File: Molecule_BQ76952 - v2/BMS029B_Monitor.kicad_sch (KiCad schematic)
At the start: 108 parts, among them J2 PEC05SAAN, J6 87898-0304, J7 87898-0304, Q1 FCX495TA, U1 bq76952PFBT

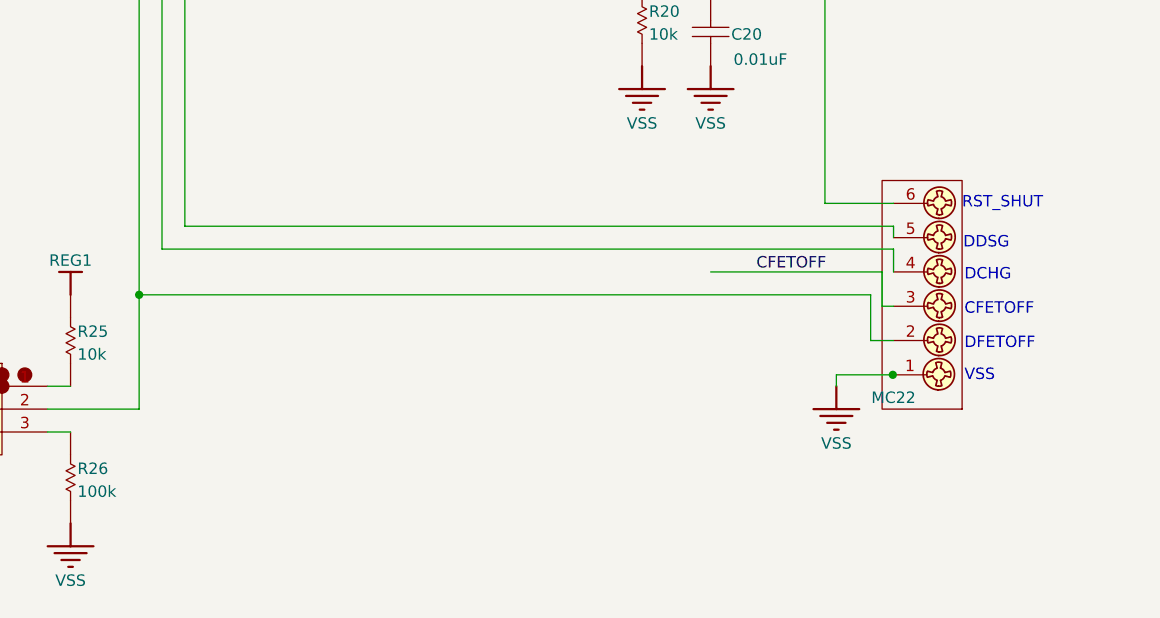
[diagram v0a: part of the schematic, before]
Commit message: Final production
Updated sizing and bug fixes
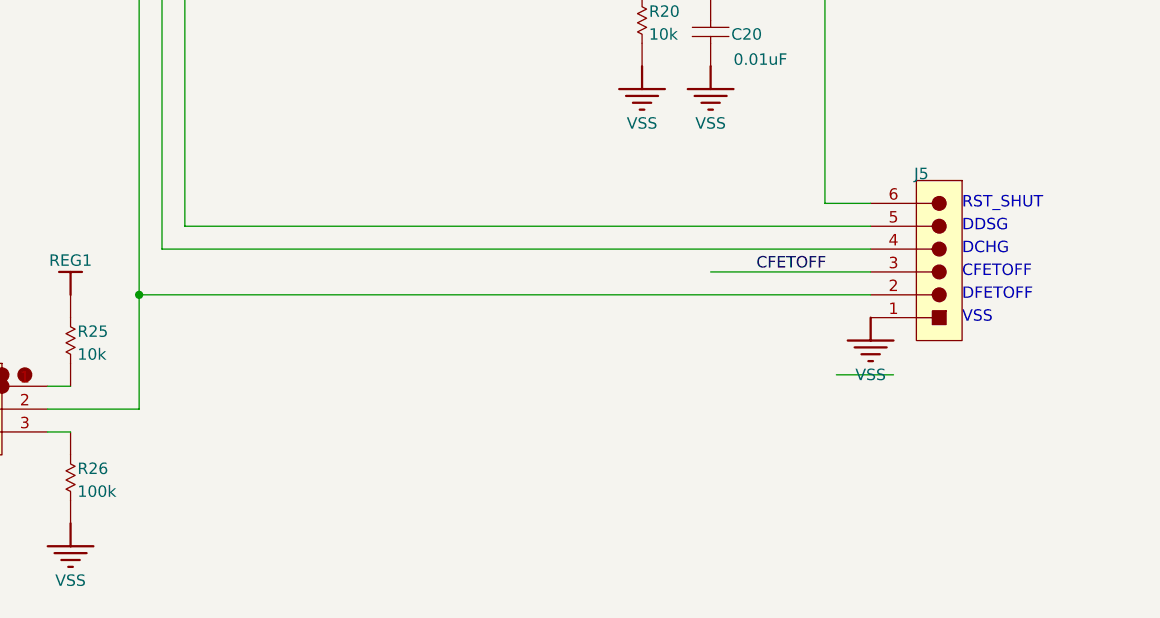
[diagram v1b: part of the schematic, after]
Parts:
- removed MC22: ~, Kales_Custom_Footprints:ADOM_MEDIUM_HEADER_6, symbol Kales_Custom_Symbols:Adom_Machine_Contact
- added J5: PEC06SAAN, Kales_Custom_Footprints:ADOM_MEDIUM_HEADER_6, symbol Altium Vault - TI:root_2_mirrored_Header_6x1_Altium Vault - TI
- J2: footprint Sullins_PxC05SAAN -> Kales_Custom_Footprints:ADOM_MEDIUM_HEADER_5
- J6, J7: footprint Molex_87898-0304 -> Adom Footprint Library:ADOM_JUMPER_4x2_3Way_Selector
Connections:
- net CFETOFF: now also J5.3
- net DCHG: now also J5.4
- net DDSG: now also J5.5
- net DFETOFF: now also J5.2
- net RST_SHUT: now also J5.6
- net VSS: now also J5.1
